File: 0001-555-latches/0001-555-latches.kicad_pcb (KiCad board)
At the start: 2 copper layers, 88 x 75 mm, 37 parts, among them J1 DC_IN, J2 ASTBL_OUT, J3 BSTBL_OUT, J4 MSTBL_OUT, SW1 SW_Push, SW2 SW_Push, SW3 SW_Push, U1 NE555P, U2 NE555P, U3 NE555P

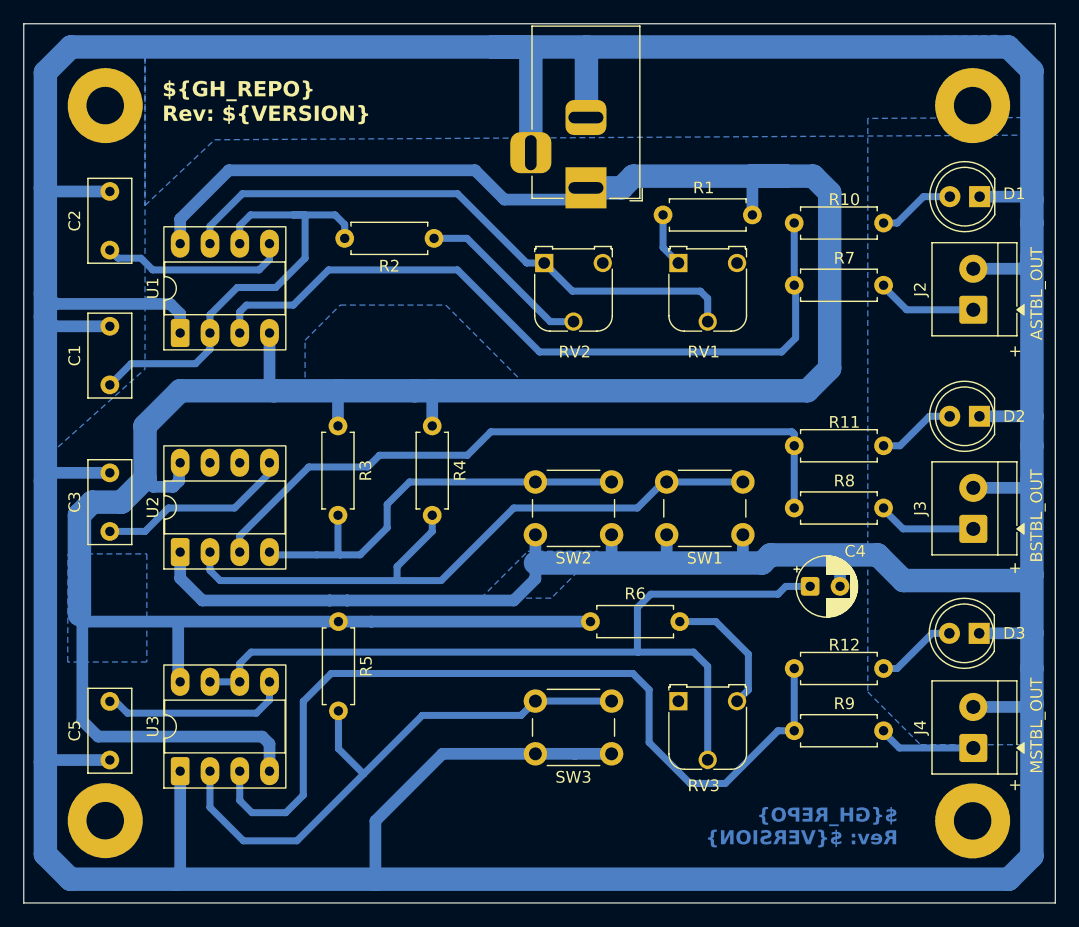
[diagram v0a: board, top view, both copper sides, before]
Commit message: Update labels on PCB
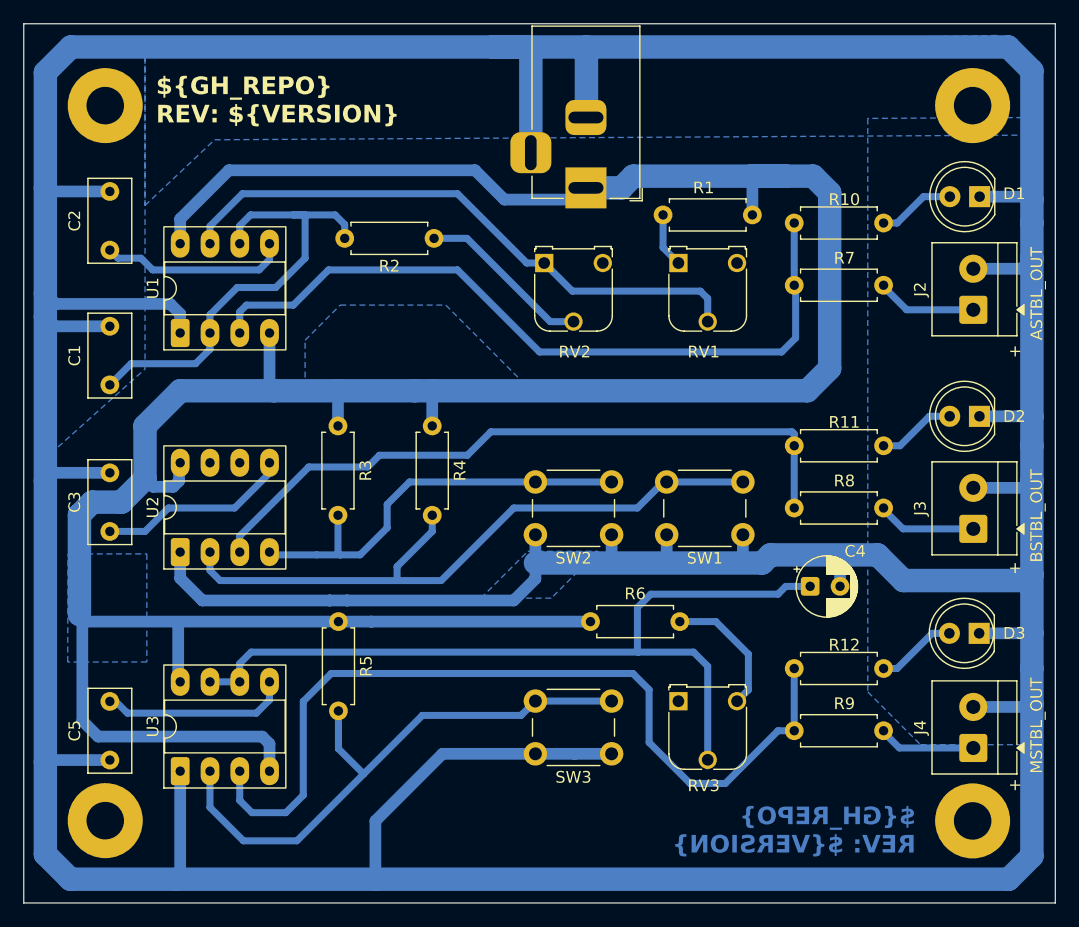
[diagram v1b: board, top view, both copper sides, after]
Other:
- board text added: "${GH_REPO} REV: ${VERSION}"
- board text removed: "${GH_REPO} Rev: ${VERSION}"
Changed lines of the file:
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@@
 		)
 	)
-	(property "GH_REPO" "github.com/mc-hw/0001")
-	(property "VERSION" "1.0.0")
+	(property "GH_REPO" "GITHUB.COM/MC-HW/0001")
+	(property "VERSION" "1.0.1")
 	(net 0 "")
 	(net 1 "GND")
@@
 		(layer "Edge.Cuts")
 	)
-	(gr_text "${GH_REPO}\nRev: ${VERSION}"
-		(at 175.57 131.14 0)
+	(gr_text "${GH_REPO}\nREV: ${VERSION}"
+		(at 177.1 131.88 0)
 		(layer "B.Cu")
 		(effects
 			(font
-				(size 1.2 1.2)
-				(thickness 0.24)
+				(size 1.5 1.5)
+				(thickness 0.3)
+				(bold yes)
+			)
+			(justify left bottom mirror)
+		)
+	)
+	(gr_text "${GH_REPO}\nREV: ${VERSION}"
+		(at 142.77 69.39 0)
+		(layer "B.Mask")
+		(effects
+			(font
+				(size 1.5 1.5)
+				(thickness 0.3)
 				(bold yes)
 			)
@@
 		)
 	)
-	(gr_text "${GH_REPO}\nRev: ${VERSION}"
-		(at 112.813608 69.44284 0)
+	(gr_text "${GH_REPO}\nREV: ${VERSION}"
+		(at 112.28 69.6 0)
 		(layer "F.SilkS")
 		(effects
 			(font
-				(size 1.3 1.3)
-				(thickness 0.26)
+				(size 1.5 1.5)
+				(thickness 0.3)
 				(bold yes)
 			)
